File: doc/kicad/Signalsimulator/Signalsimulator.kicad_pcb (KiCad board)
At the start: 2 copper layers, 38.1 x 38.1 mm, 14 parts, among them J1 Conn_02x03_Odd_Even

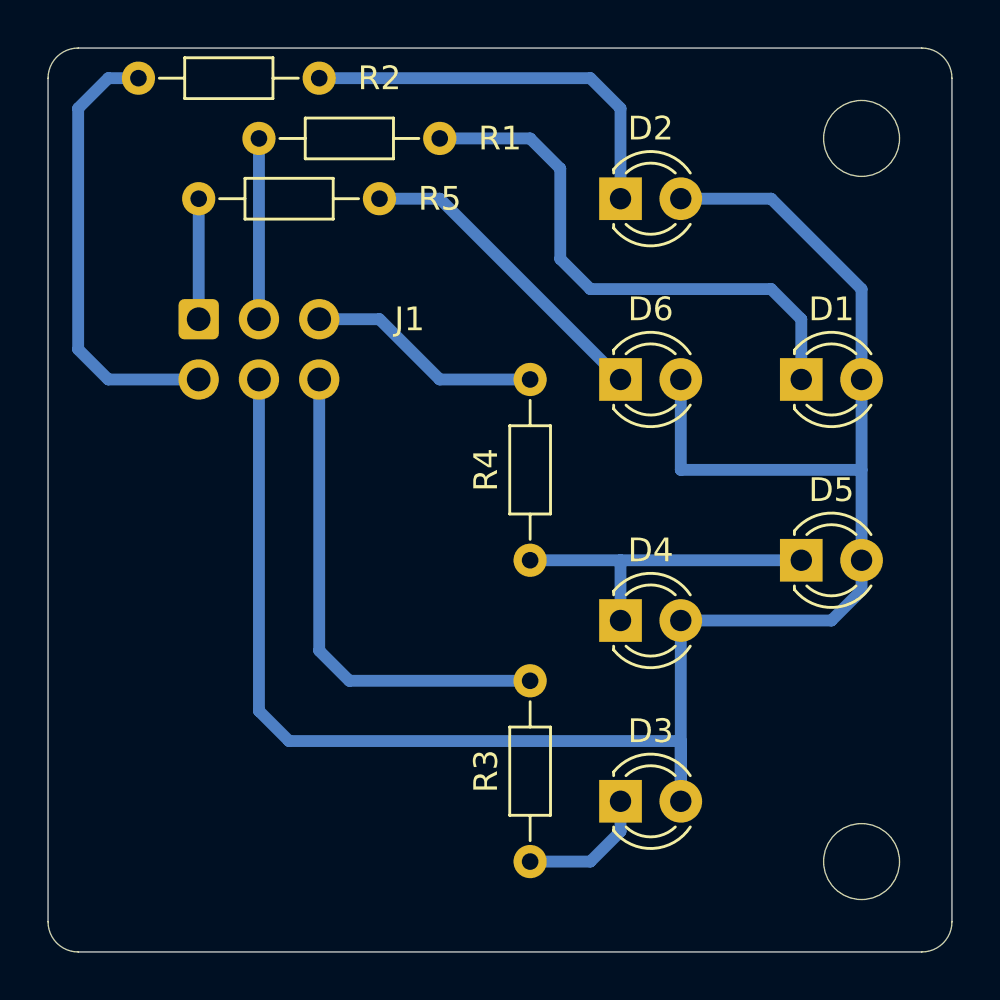
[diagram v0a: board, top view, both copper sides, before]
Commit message: Aufgeräumt
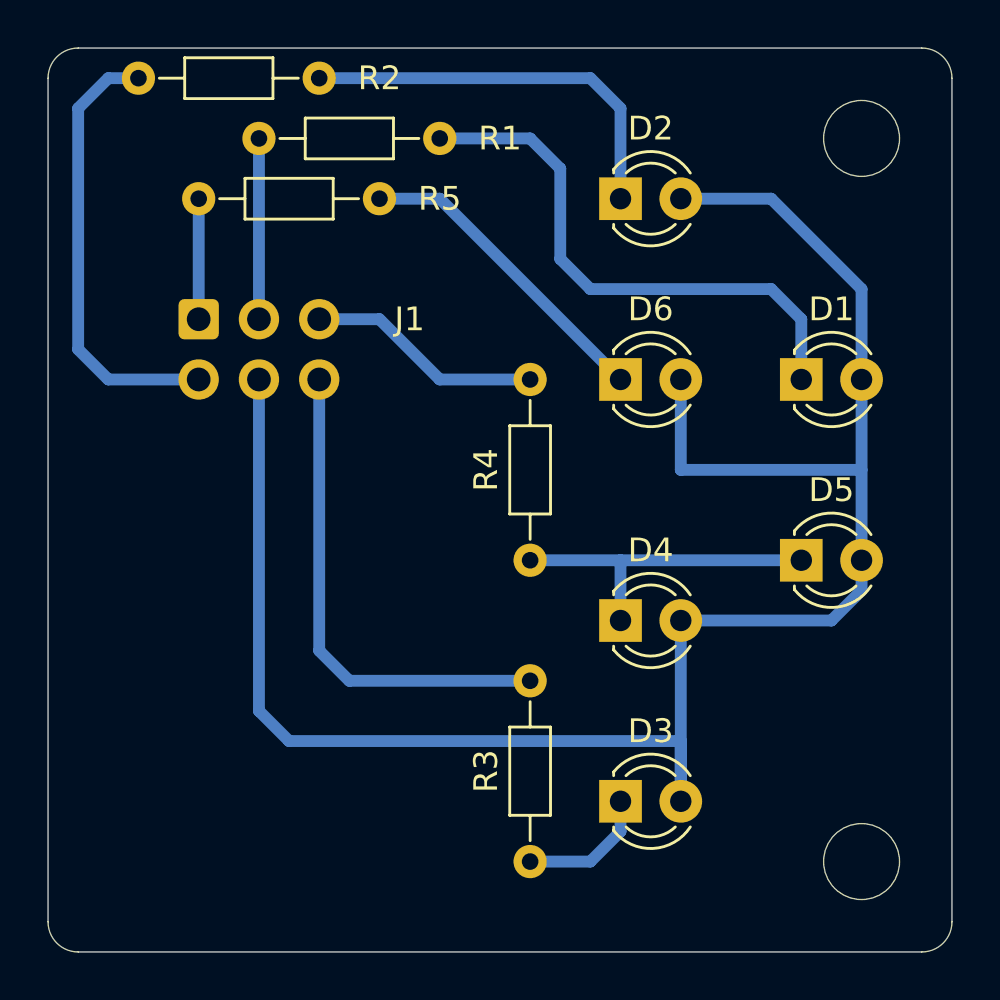
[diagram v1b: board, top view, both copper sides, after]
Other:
- net class Default removed
